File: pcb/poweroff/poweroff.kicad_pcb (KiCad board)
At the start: 2 copper layers, 39.4 x 40.6 mm, 14 parts, among them P1 CONN_01X03, P2 CONN_01X02, P3 CONN_01X02, Q1 BC547, Q2 BC547

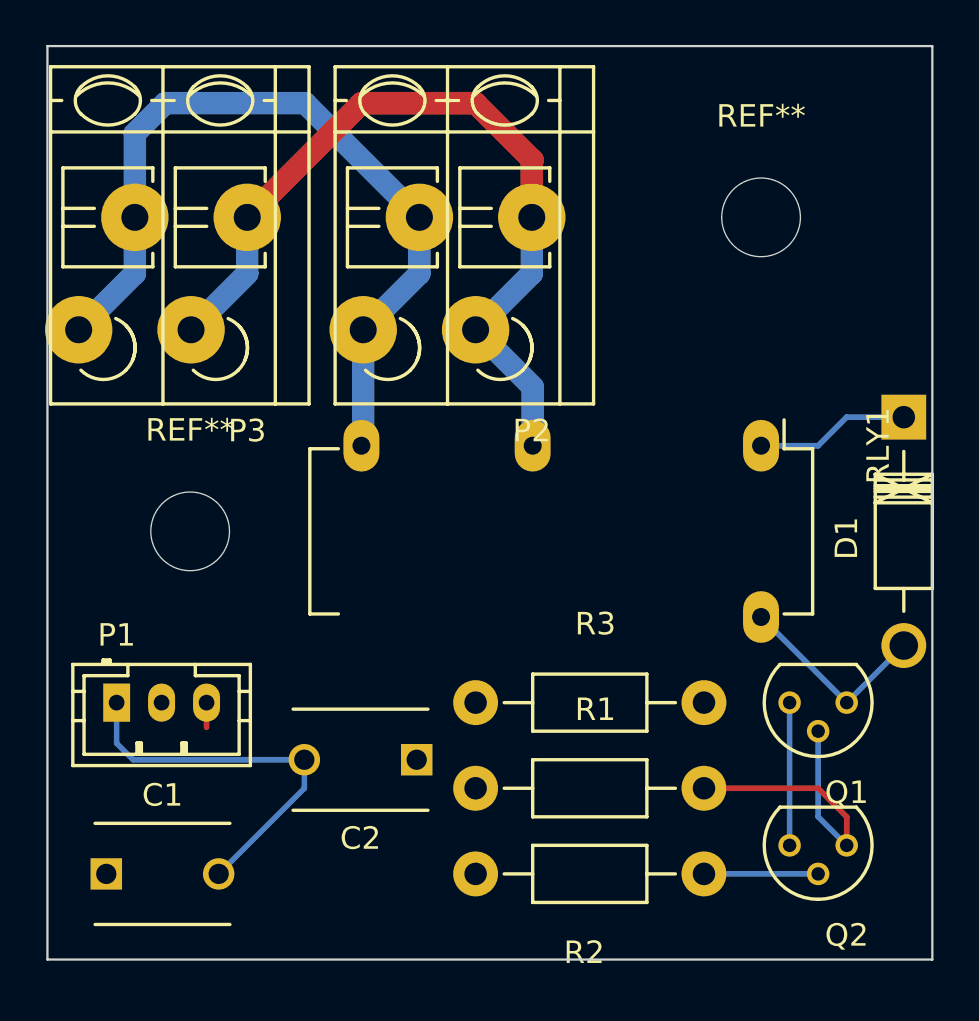
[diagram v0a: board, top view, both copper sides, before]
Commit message: Reduce size.
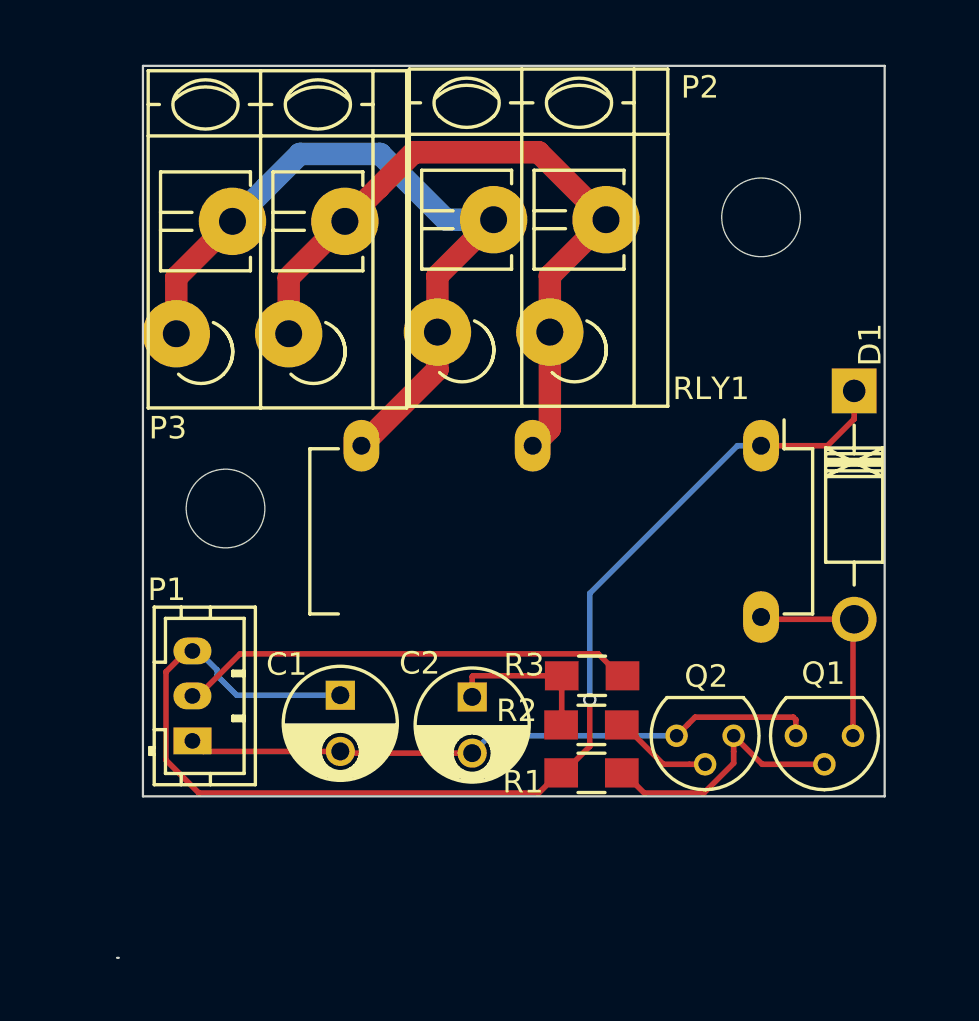
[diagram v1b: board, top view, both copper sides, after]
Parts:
- C1, C2: footprint Capacitors_ThroughHole:C_Disc_D6_P5 -> Capacitors_ThroughHole:C_Radial_D5_L6_P2.5
- R1, R2, R3: footprint Resistors_ThroughHole:Resistor_Horizontal_RM10mm -> Resistors_SMD:R_0805_HandSoldering
- moved C1 13.1 mm to (171.8, 100.0), turned to 270 degrees
- moved R2 8.31 mm to (183.0, 101.3)
- moved Q2 7.01 mm to (189.3, 101.8)
- moved R3 5.32 mm to (183.0, 99.1)
- moved R1 5.20 mm to (183.0, 103.5)
- moved P3 4.35 mm to (172.0, 78.9)
- moved P1 3.78 mm to (165.2, 102.0), turned to 90 degrees
- moved C2 3.73 mm to (177.6, 100.1), turned to 270 degrees
- moved P2 3.30 mm to (183.6, 78.8)
- moved D1 2.50 mm to (194.6, 86.5)
- moved H1 1.87 mm to (166.7, 91.7)
- moved Q1 1.50 mm to (194.6, 101.8)
- renumbered REF** to H1, REF** to H2
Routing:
- net +5V: track 7.98 -> 56.4 mm, vias 0 -> 1
- net Net-(P1-Pad2): track 0.00 -> 20.3 mm
- net Net-(C2-Pad1): track 0.00 -> 7.10 mm
- net Net-(P2-Pad1): track 36.7 -> 31.6 mm
- net GND: track 23.5 -> 28.5 mm
- net Net-(P2-Pad2): track 36.3 -> 32.7 mm
- net Net-(Q1-Pad2): track 13.8 -> 11.7 mm
- net Net-(Q2-Pad2): track 5.08 -> 4.43 mm
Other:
- board size 39.4 x 40.6 mm -> 34.2 x 39.7 mm
- net class Mains: clearance 3 -> 1
